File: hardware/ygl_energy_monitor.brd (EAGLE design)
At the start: 73.5 x 52 mm, 5 parts, among them IC1 ACS750LCA-050

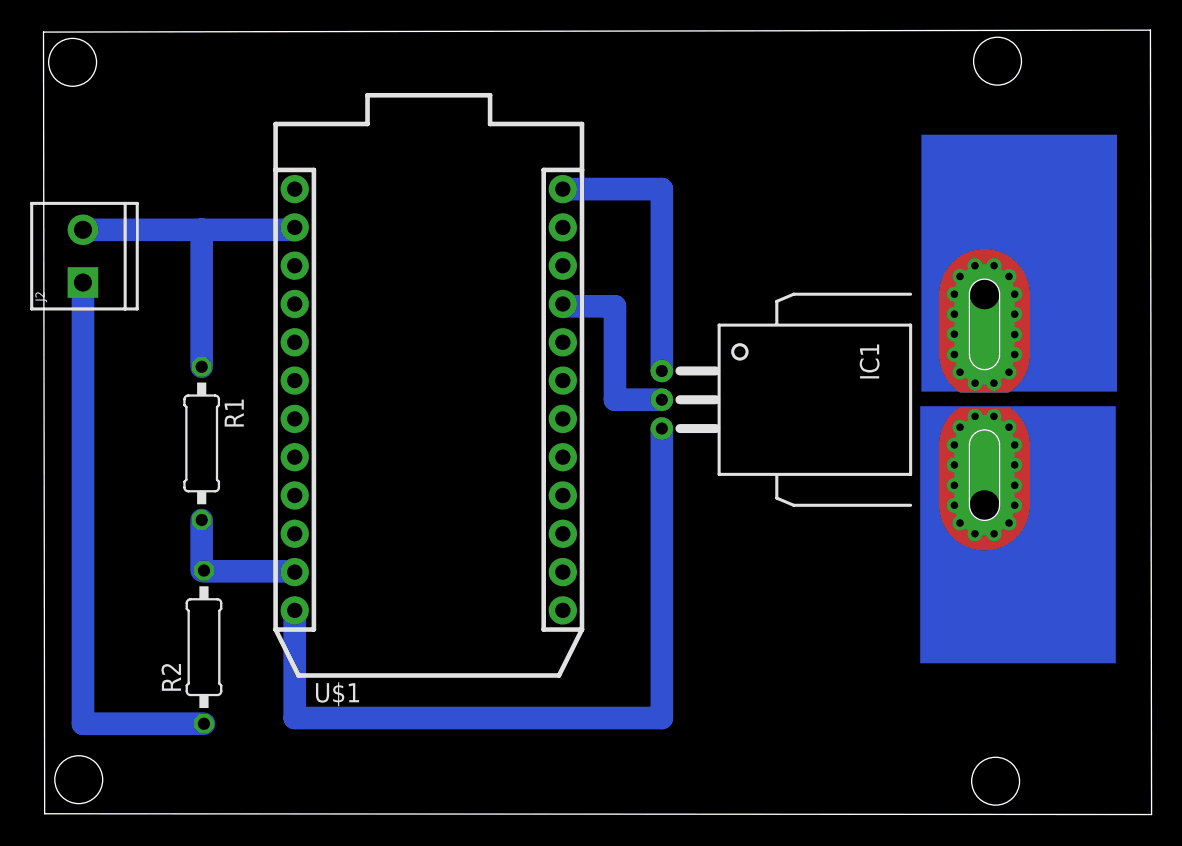
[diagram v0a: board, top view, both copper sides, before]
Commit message: fuck braze!
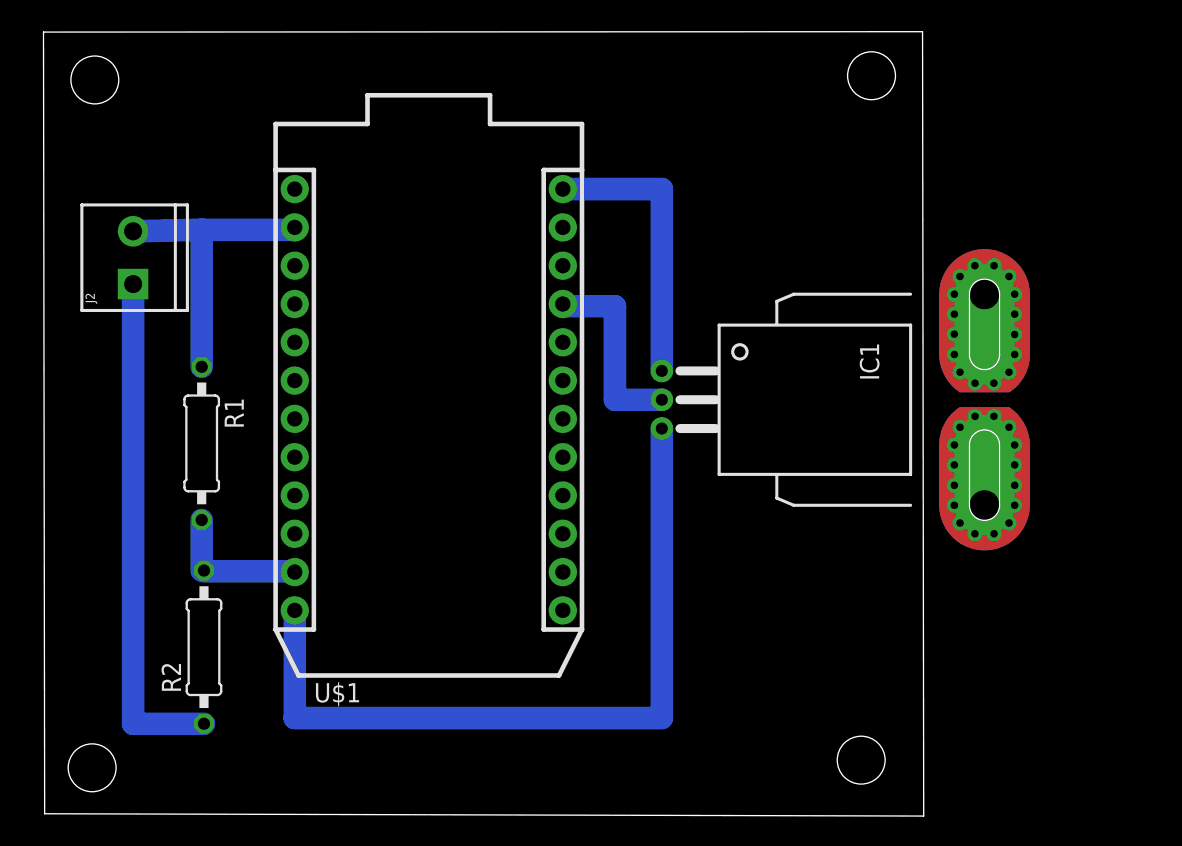
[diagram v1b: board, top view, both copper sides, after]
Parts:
- moved J2 3.33 mm to (5.79, 43.7)
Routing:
- net N$5: track 37.3 -> 33.9 mm
- net N$4: track 23.3 -> 20.0 mm
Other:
- board size 73.5 x 52 mm -> 58.4 x 52 mm
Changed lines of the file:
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@@
 <board>
 <plain>
-<wire x1="-0.0762" y1="8.6106" x2="73.3352" y2="8.5598" width="0" layer="20"/>
-<wire x1="73.3352" y1="8.5598" x2="73.259" y2="60.5792" width="0" layer="20"/>
-<wire x1="73.259" y1="60.5792" x2="-0.1524" y2="60.4522" width="0" layer="20"/>
+<wire x1="-0.0762" y1="8.6106" x2="58.2222" y2="8.4582" width="0" layer="20"/>
+<wire x1="58.2222" y1="8.4582" x2="58.146" y2="60.4776" width="0" layer="20"/>
+<wire x1="58.146" y1="60.4776" x2="-0.1524" y2="60.4522" width="0" layer="20"/>
 <wire x1="-0.1524" y1="60.4522" x2="-0.0762" y2="8.6106" width="0" layer="20"/>
-<hole x="1.778" y="58.4454" drill="3.175"/>
-<hole x="2.1844" y="10.8712" drill="3.175"/>
-<hole x="62.992" y="10.7696" drill="3.175"/>
-<hole x="63.119" y="58.5216" drill="3.175"/>
-<rectangle x1="0.6096" y1="58.0898" x2="0.8382" y2="58.2168" layer="16"/>
-<rectangle x1="57.9882" y1="18.5928" x2="70.9676" y2="35.6362" layer="16"/>
-<rectangle x1="58.0644" y1="36.6014" x2="71.0438" y2="53.6448" layer="16"/>
-<rectangle x1="59.055" y1="36.6014" x2="65.5574" y2="49.276" layer="45"/>
-<rectangle x1="59.055" y1="22.987" x2="65.5574" y2="35.6616" layer="45"/>
+<hole x="3.2512" y="57.277" drill="3.175"/>
+<hole x="3.0734" y="11.6586" drill="3.175"/>
+<hole x="54.0766" y="12.1666" drill="3.175"/>
+<hole x="54.7624" y="57.5564" drill="3.175"/>
 </plain>
 <attributes>
@@
 <elements>
 <element name="U$1" library="Spark" package="PHOTON" value="PHOTON_WITH_HEADERS" x="15.24" y="17.78"/>
-<element name="J2" library="SparkFun-Connectors" package="SCREWTERMINAL-3.5MM-2" value="" x="2.4638" y="43.8404" rot="R90">
-<attribute name="PROD_ID" value="CONN-08399" x="2.4638" y="43.8404" size="1.778" layer="27" rot="R90" display="off"/>
+<element name="J2" library="SparkFun-Connectors" package="SCREWTERMINAL-3.5MM-2" value="" x="5.7912" y="43.7388" rot="R90">
+<attribute name="PROD_ID" value="CONN-08399" x="5.7912" y="43.7388" size="1.778" layer="27" rot="R90" display="off"/>
 </element>
 <element name="R2" library="resistor" library_urn="urn:adsk.eagle:library:348" package="0207/10" package3d_urn="urn:adsk.eagle:package:25939/1" value="" x="10.4902" y="19.6596" rot="R90"/>
@@
 <contactref element="R1" pad="1"/>
 <contactref element="J2" pad="2"/>
-<wire x1="2.4638" y1="47.3404" x2="10.3378" y2="47.3404" width="1.5" layer="16"/>
+<wire x1="5.7912" y1="47.2388" x2="10.3378" y2="47.3404" width="1.5" layer="16"/>
 <wire x1="10.3378" y1="47.3404" x2="16.51" y2="47.3404" width="1.5" layer="16"/>
 <wire x1="16.51" y1="47.3404" x2="16.51" y2="47.498" width="0.6096" layer="16"/>
@@
 <contactref element="J2" pad="1"/>
 <contactref element="R2" pad="1"/>
-<wire x1="2.4638" y1="43.8404" x2="2.4638" y2="14.5796" width="1.5" layer="16"/>
-<wire x1="2.4638" y1="14.5796" x2="10.4902" y2="14.5796" width="1.5" layer="16"/>
+<wire x1="5.7912" y1="43.7388" x2="5.7912" y2="14.5796" width="1.5" layer="16"/>
+<wire x1="5.7912" y1="14.5796" x2="10.4902" y2="14.5796" width="1.5" layer="16"/>
 </signal>
 </signals>
